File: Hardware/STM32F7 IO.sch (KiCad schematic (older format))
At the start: 19 parts, among them U16 STM32F765ZGT6

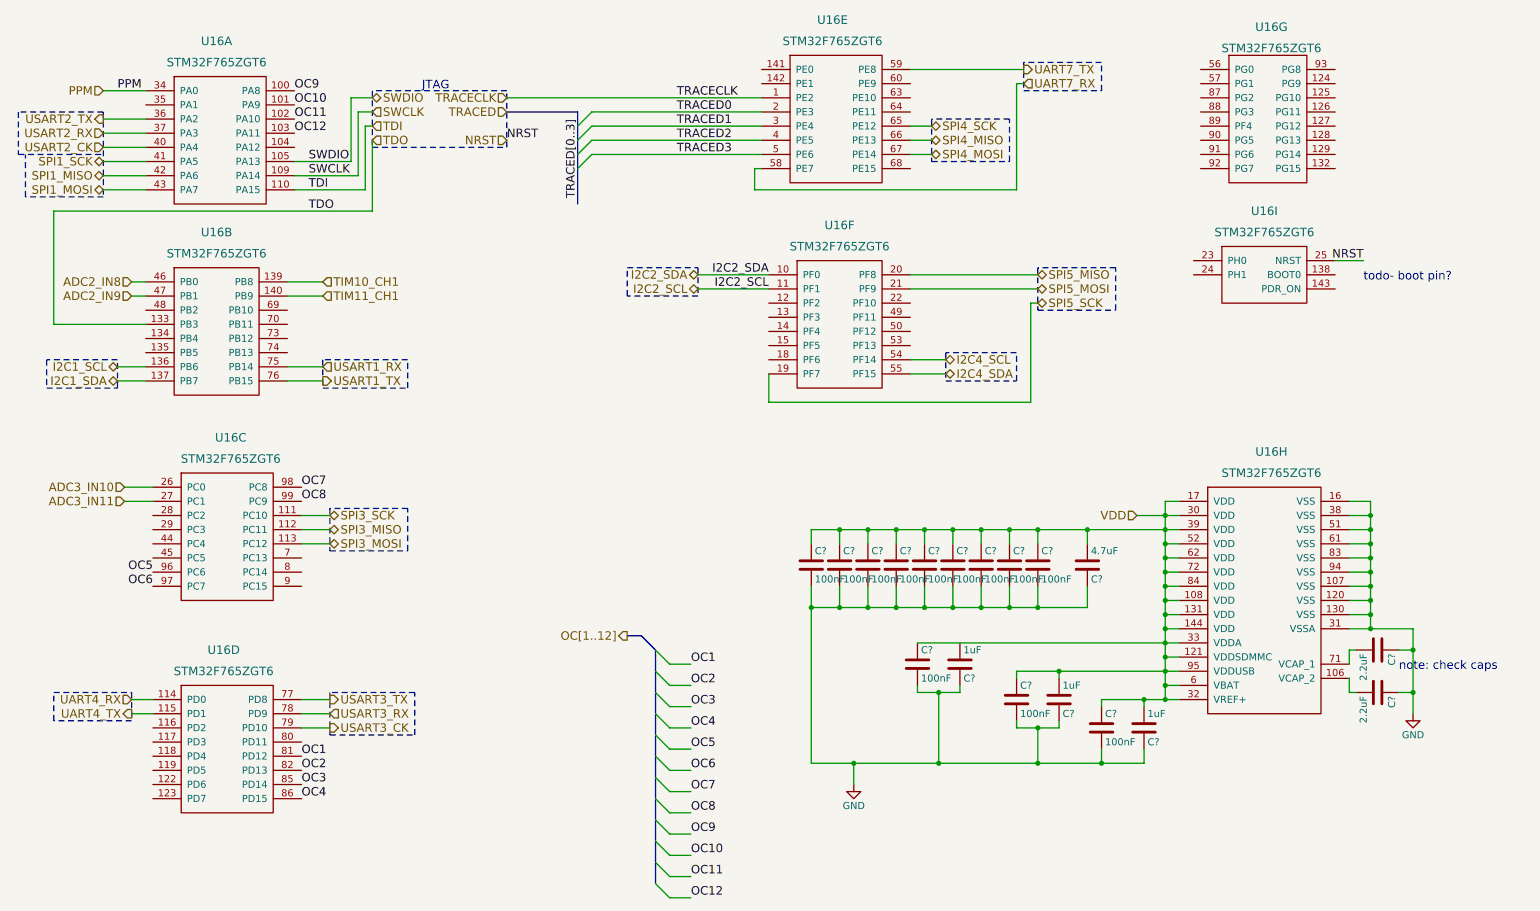
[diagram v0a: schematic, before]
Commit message: Reconfiguring pinout round 2
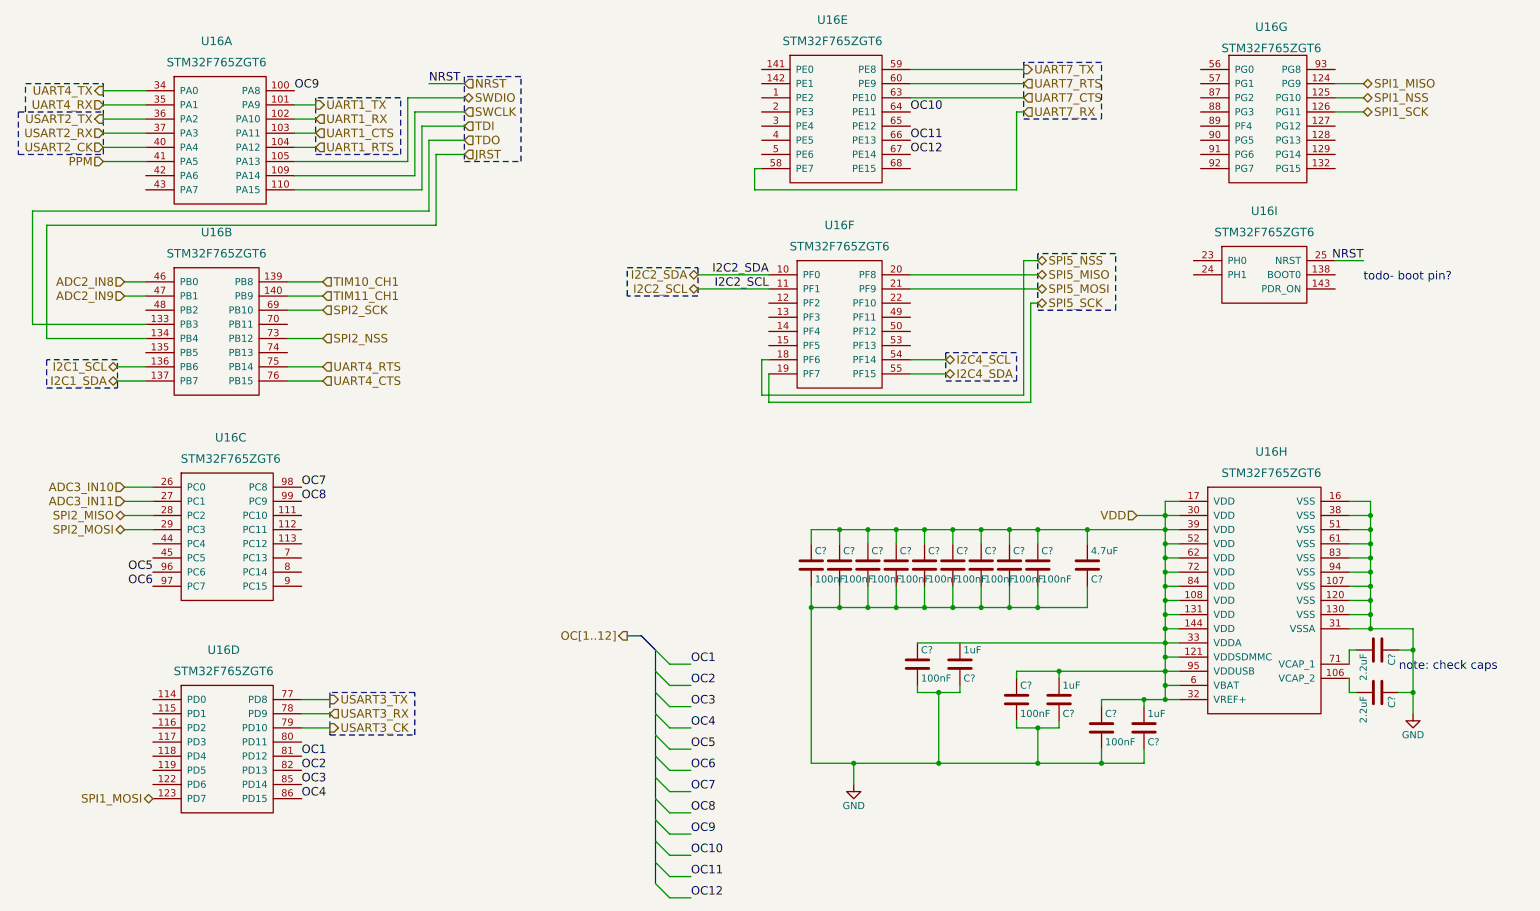
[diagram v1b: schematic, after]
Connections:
- net SPI4_MISO is gone; now on net OC11: U16.66 (PE13)
- net SPI4_MOSI is gone; now on net OC12: U16.67 (PE14)
- net OC10: now also U16.64 (PE11); no longer U16.101 (PA9)
- net OC11: no longer U16.102 (PA10)
- net OC12: no longer U16.103 (PA11)
- net PPM: now also U16.41 (PA5); no longer U16.34 (PA0)
- net SPI1_MISO: now also U16.124 (PG9); no longer U16.42 (PA6)
- net SPI1_MOSI: now also U16.123 (PD7); no longer U16.43 (PA7)
- net SPI1_SCK: now also U16.126 (PG11); no longer U16.41 (PA5)
- net UART4_RX: now also U16.35 (PA1); no longer U16.114 (PD0)
- net UART4_TX: now also U16.34 (PA0); no longer U16.115 (PD1)
- net UART1_RTS: now reaches U16.104 (PA12)
- net JRST: now reaches U16.134 (PB4)
- net SPI2_SCK: now reaches U16.69 (PB10)
- net SPI2_NSS: now reaches U16.73 (PB12)
- net SPI2_MISO: now reaches U16.28 (PC2)
- net SPI2_MOSI: now reaches U16.29 (PC3)
- net UART7_RTS: now reaches U16.60 (PE9)
- net UART7_CTS: now reaches U16.63 (PE10)
- net SPI5_NSS: now reaches U16.18 (PF6)
- net SPI1_NSS: now reaches U16.125 (PG10)
- net SPI3_MISO: no longer names the net of U16.112 (PC11)
- net SPI3_MOSI: no longer names the net of U16.113 (PC12)
- net SPI3_SCK: no longer names the net of U16.111 (PC10)
- net SPI4_SCK: no longer names the net of U16.65 (PE12)
- net TRACECLK: no longer names the net of U16.1 (PE2)
- net TRACED0: no longer names the net of U16.2 (PE3)
- net TRACED1: no longer names the net of U16.3 (PE4)
- net TRACED2: no longer names the net of U16.4 (PE5)
- net TRACED3: no longer names the net of U16.5 (PE6)
- net USART1_RX renamed UART4_RTS
- net USART1_TX renamed UART4_CTS
- new net UART1_CTS: U16.103 (PA11)
- new net UART1_RX: U16.102 (PA10)
- new net UART1_TX: U16.101 (PA9)
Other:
- note removed: "JTAG"
